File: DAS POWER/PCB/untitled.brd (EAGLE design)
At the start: 154 x 83.1 mm, 66 parts, among them J1 10118193-0001LF, J2 22-27-2041-04, Q1 12MHz, Q2 MMBT3904, Q3 MMBT3904, U1 CH340G, U2 AMS1117, U3 ESP32-WROOM-32D, X1 MSTBA2, X2 MSTBA6, X3 MSTBA6, X4 MSTBA6, X5 MSTBA2, X6 MSTBA2, X7 MSTBA2, X8 MSTBA2, X9 22-23-2021

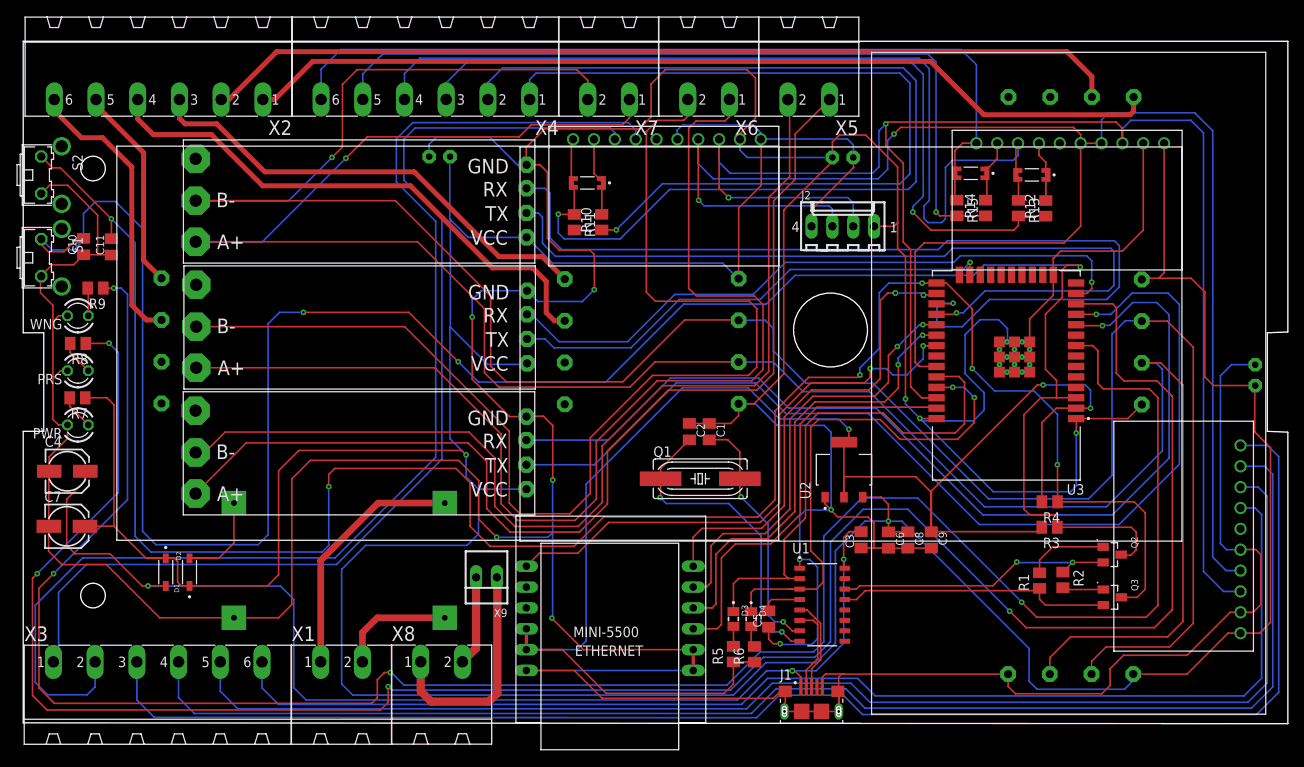
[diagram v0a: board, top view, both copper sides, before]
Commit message: revisi final tanggal 21/02.2023
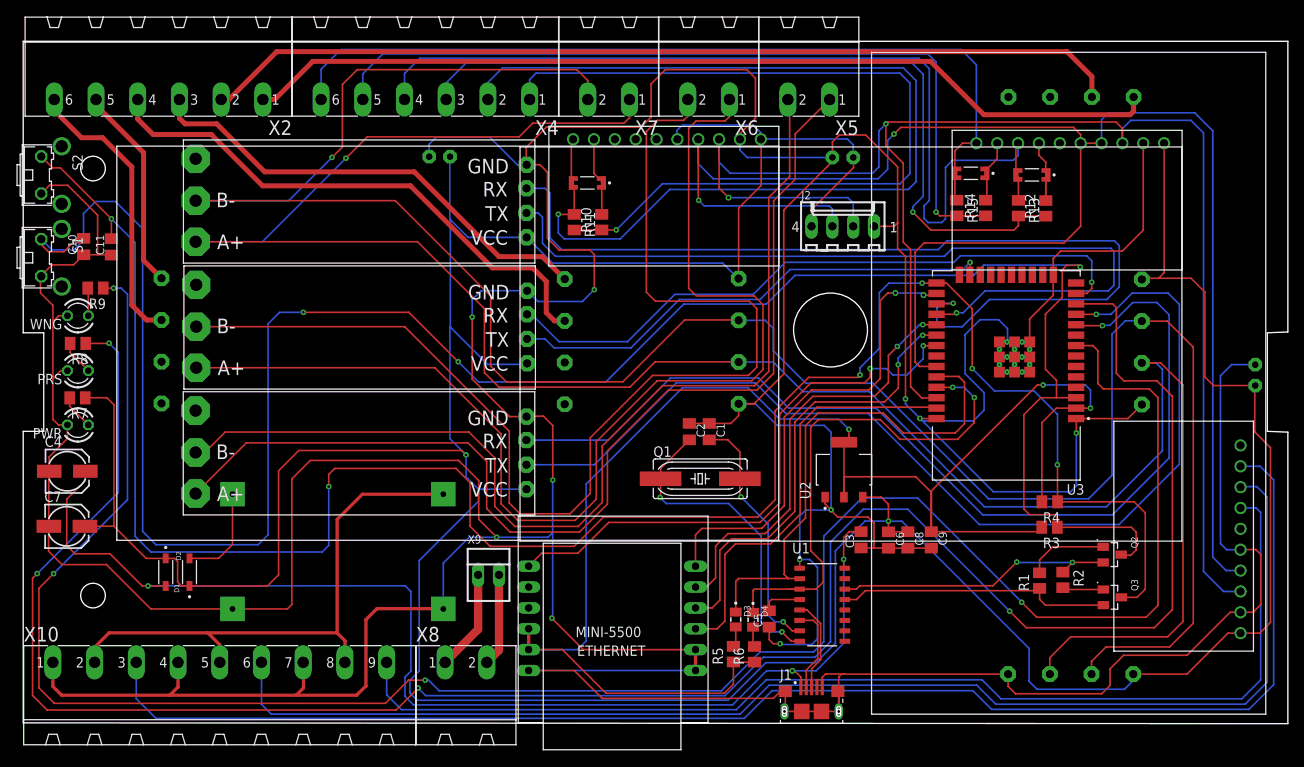
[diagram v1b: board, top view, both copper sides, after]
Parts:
- removed X1: MSTBA2, con-phoenix-508:MSTBA2
- removed X3: MSTBA6, con-phoenix-508:MSTBA6
- added X10: MSTBA9, con-phoenix-508:MSTBA9
- moved X8 2.97 mm to (59.1, 124.4)
- moved MINI1 1.09 mm to (56.3, 151.3)
- moved X9 0.39 mm to (61.9, 140.2), turned to 0 degrees
- moved D3 0.29 mm to (92.0, 134.7)
- moved U$1 0.28 mm to (88.6, 122.2)
- moved D4 0.24 mm to (94.1, 134.7)
- moved C5 0.07 mm to (96.0, 134.8)
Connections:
- removed net A0+: ADS1.A0, X3.6
- removed net A0-: ADS1.A1, X3.5
- removed net A1+: ADS1.A2, X3.4
- removed net A1-: ADS1.A3, X3.3
- removed net A2+: ADS2.A0, X3.2
- removed net A2-: ADS2.A1, X3.1
- removed net N$3: MINI1.IN+, X1.1
- removed net N$5: MINI1.IN-, X1.2
- new net +12V: MINI1.IN+, X10.2, X10.5, X10.8
- new net A0: ADS1.A2, X10.3
- new net A1: ADS1.A1, X10.6
- new net A2: ADS1.A0, X10.9
- net GND: now also MINI1.IN-, X10.1, X10.4, X10.7
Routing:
- net A1-: track 181.7 -> 0.00 mm
- net A0: track 0.00 -> 177.2 mm
- net A1+: track 171.9 -> 0.00 mm
- net A0-: track 161.6 -> 0.00 mm
- net A1: track 0.00 -> 158.0 mm
- net A0+: track 151.6 -> 0.00 mm
- net A2+: track 149.2 -> 0.00 mm
- net A2: track 0.00 -> 137.6 mm
- net A2-: track 130.3 -> 0.00 mm
- net GND: track 787.0 -> 868.3 mm
- net +12V: track 0.00 -> 68.3 mm
- net N$3: track 30.4 -> 0.00 mm
- net OUT+: track 498.5 -> 480.6 mm
- net N$17: track 28.0 -> 12.3 mm
- net N$5: track 14.3 -> 0.00 mm
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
